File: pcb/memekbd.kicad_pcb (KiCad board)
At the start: 2 copper layers, 134.1 x 130.9 mm, 209 parts, among them J1 AudioJack4, J2 AudioJack4, SW1 SW_Push, SW10 SW_Push, SW11 SW_Push, SW12 SW_Push, SW13 SW_Push, SW14 SW_Push, SW15 SW_Push, SW16 SW_Push, SW17 SW_Push, SW18 SW_Push, SW19 SW_Push, SW2 SW_Push, SW20 SW_Push, SW21 SW_Push, SW22 SW_Push, SW23 SW_Push, SW24 SW_Push, SW25 SW_Push, SW26 SW_Push, SW27 SW_Push, SW28 SW_Push, SW29 SW_Push, SW3 SW_Push, SW30 SW_Push, SW31 SW_Push, SW32 SW_Push, SW33 SW_Push, SW34 SW_Push, SW35 SW_Push, SW36 SW_Push, SW37 SW_Push, SW38 SW_Push, SW39 SW_Push, SW4 SW_Push, SW40 SW_Push, SW41 SW_Push, SW42 SW_Push, SW43 SW_Push, SW44 SW_Push, SW45 SW_Push, SW46 SW_Push, SW47 SW_Push, SW48 SW_Push, SW5 SW_Push, SW6 SW_Push, SW7 SW_Push, SW8 SW_Push, SW9 SW_Push, U1 ProMicro, U2 ProMicro

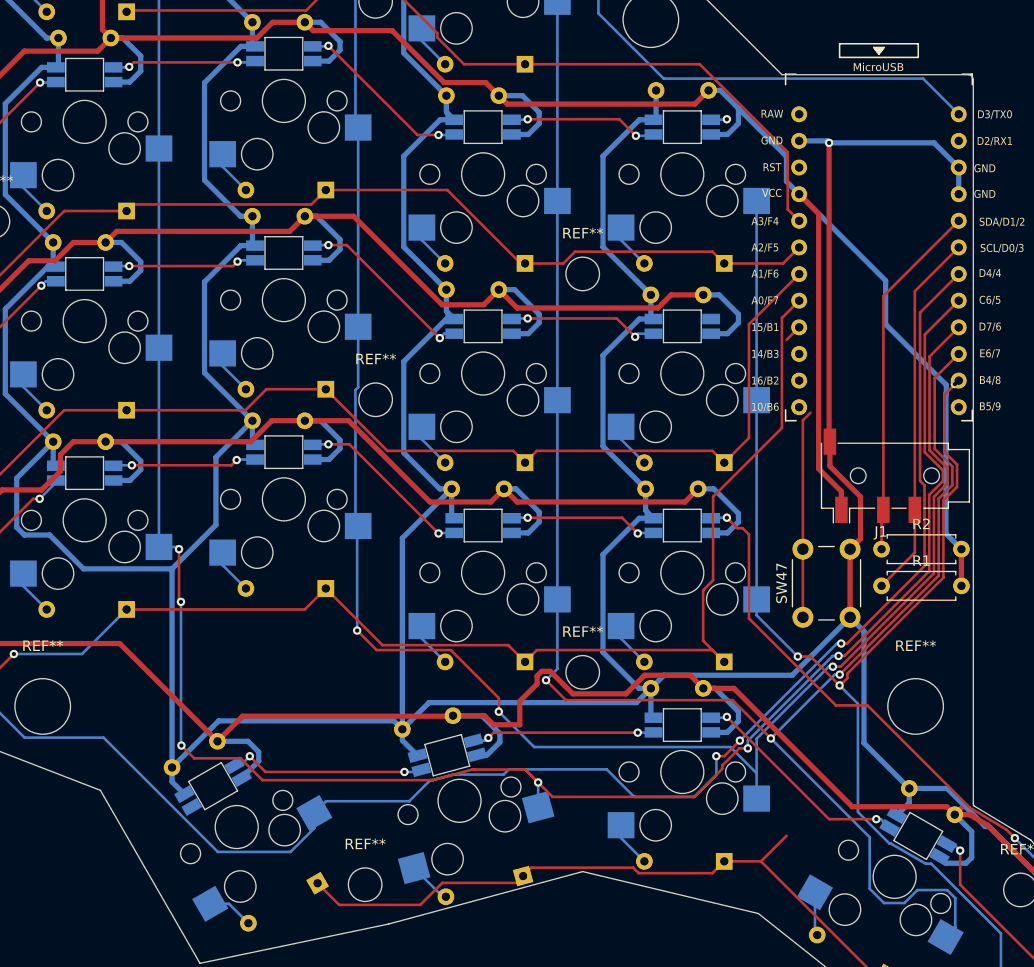
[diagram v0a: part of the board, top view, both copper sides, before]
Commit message: Routing progress
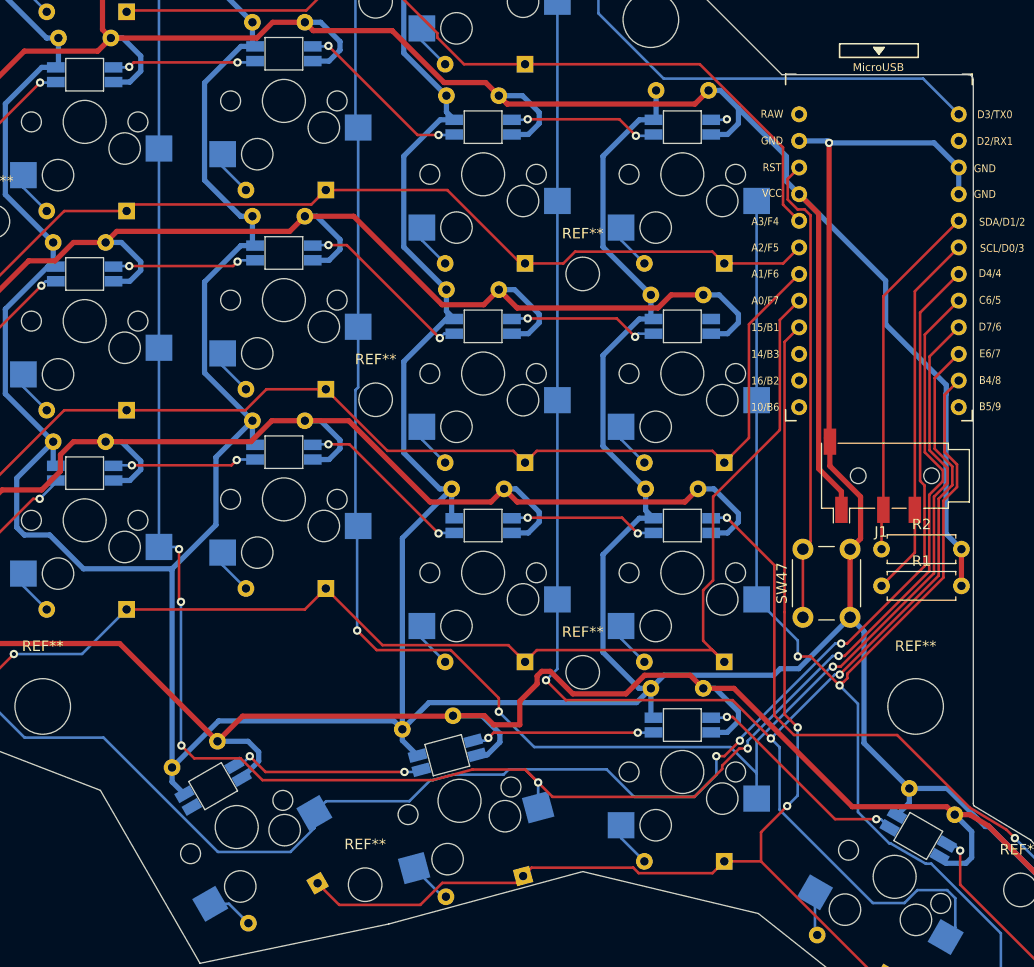
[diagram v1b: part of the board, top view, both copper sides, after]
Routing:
- net /lrow4: track 86.6 -> 134.9 mm, vias 0 -> 2
- net /lRST: track 19.8 -> 44.9 mm
- net Net-(LED22-Pad2): track 66.9 -> 70.6 mm
- net +5V: track 785.9 -> 785.0 mm
- net /lcol3: track 166.8 -> 167.5 mm
- net /lcol4: vias 3 -> 2
